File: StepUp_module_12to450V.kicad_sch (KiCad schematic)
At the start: 0 parts

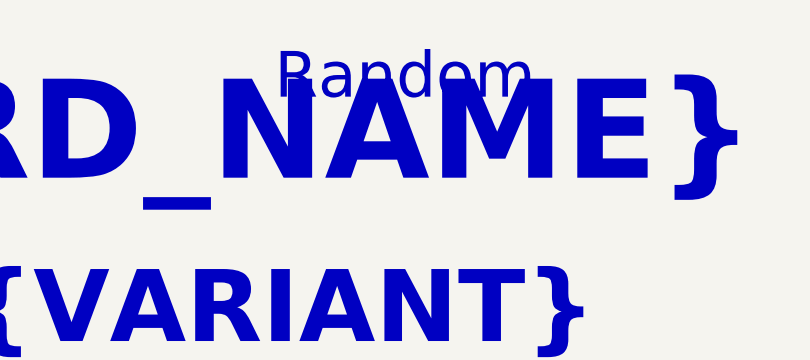
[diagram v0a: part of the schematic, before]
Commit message: DBG18
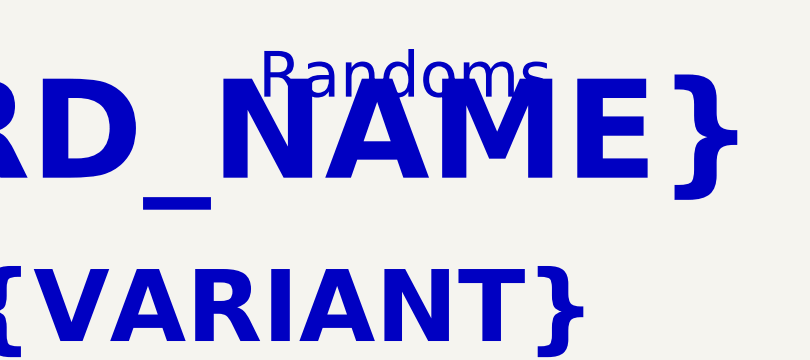
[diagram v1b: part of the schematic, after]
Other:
- note added: "Randoms"
- note removed: "Random"
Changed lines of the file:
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@@
 		)
 	)
-	(text "Random"
+	(text "Randoms"
 		(exclude_from_sim no)
 		(at 135.89 27.94 0)

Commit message: DBG17
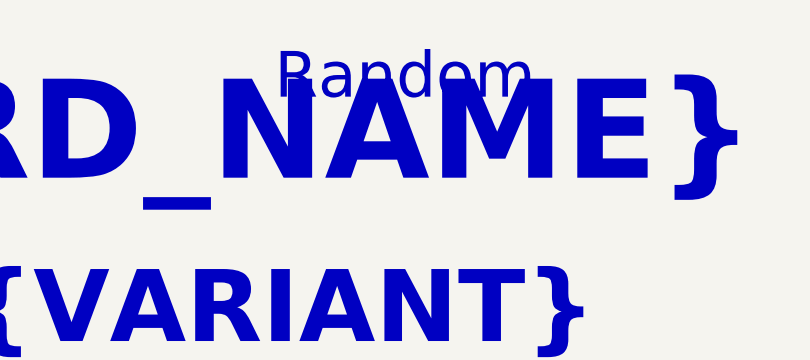
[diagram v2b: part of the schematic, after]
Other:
- note added: "Random"
- note removed: "Randoms"
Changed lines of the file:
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@@
 		)
 	)
-	(text "Randoms"
+	(text "Random"
 		(exclude_from_sim no)
 		(at 135.89 27.94 0)

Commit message: DBG13
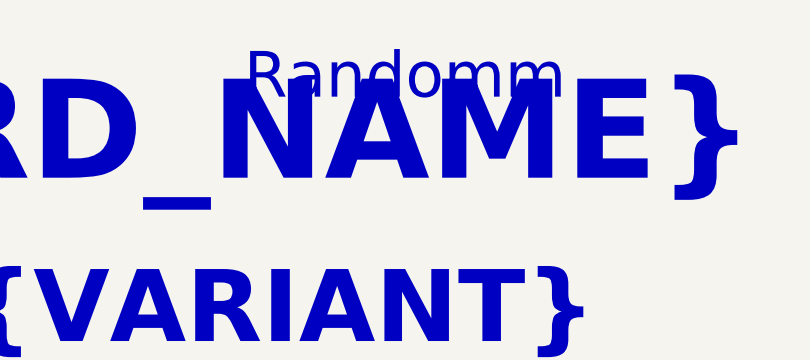
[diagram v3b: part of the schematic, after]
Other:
- note added: "Randomm"
- note removed: "Random"
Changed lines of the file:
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@@
 		)
 	)
-	(text "Random"
+	(text "Randomm"
 		(exclude_from_sim no)
 		(at 135.89 27.94 0)

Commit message: DBG14
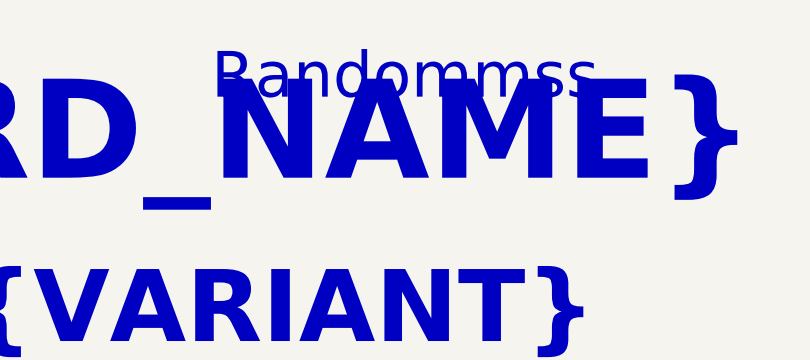
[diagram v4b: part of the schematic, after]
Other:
- note added: "Randommss"
- note removed: "Randomm"
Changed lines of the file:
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@@
 		)
 	)
-	(text "Randomm"
+	(text "Randommss"
 		(exclude_from_sim no)
 		(at 135.89 27.94 0)

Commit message: DBG15
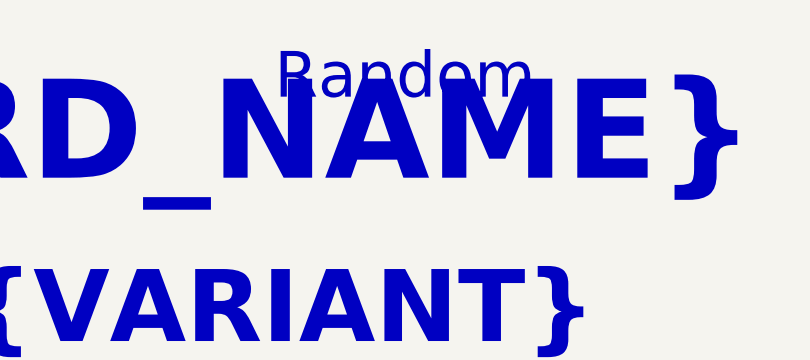
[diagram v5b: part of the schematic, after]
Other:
- note added: "Random"
- note removed: "Randommss"
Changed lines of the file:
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@@
 		)
 	)
-	(text "Randommss"
+	(text "Random"
 		(exclude_from_sim no)
 		(at 135.89 27.94 0)
